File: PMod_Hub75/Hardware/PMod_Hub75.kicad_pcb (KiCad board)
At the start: 2 copper layers, 45 x 40 mm, 16 parts, among them IC1 SN74LVC8T245DWR, IC2 SN74LVC8T245DWR, J1 Conn_02x06_Counter_Clockwise, J2 Conn_02x06_Counter_Clockwise, J3 Conn_02x08_Counter_Clockwise

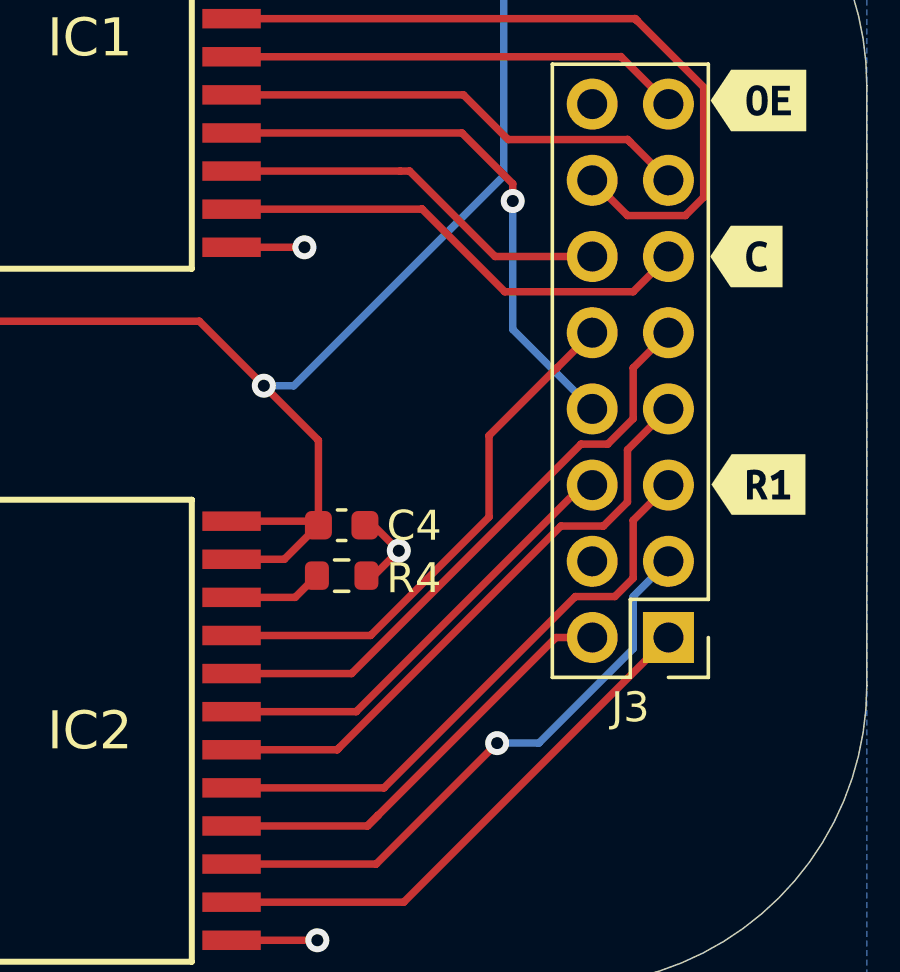
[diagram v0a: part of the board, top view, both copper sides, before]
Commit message: Fix design rules issues in pcb
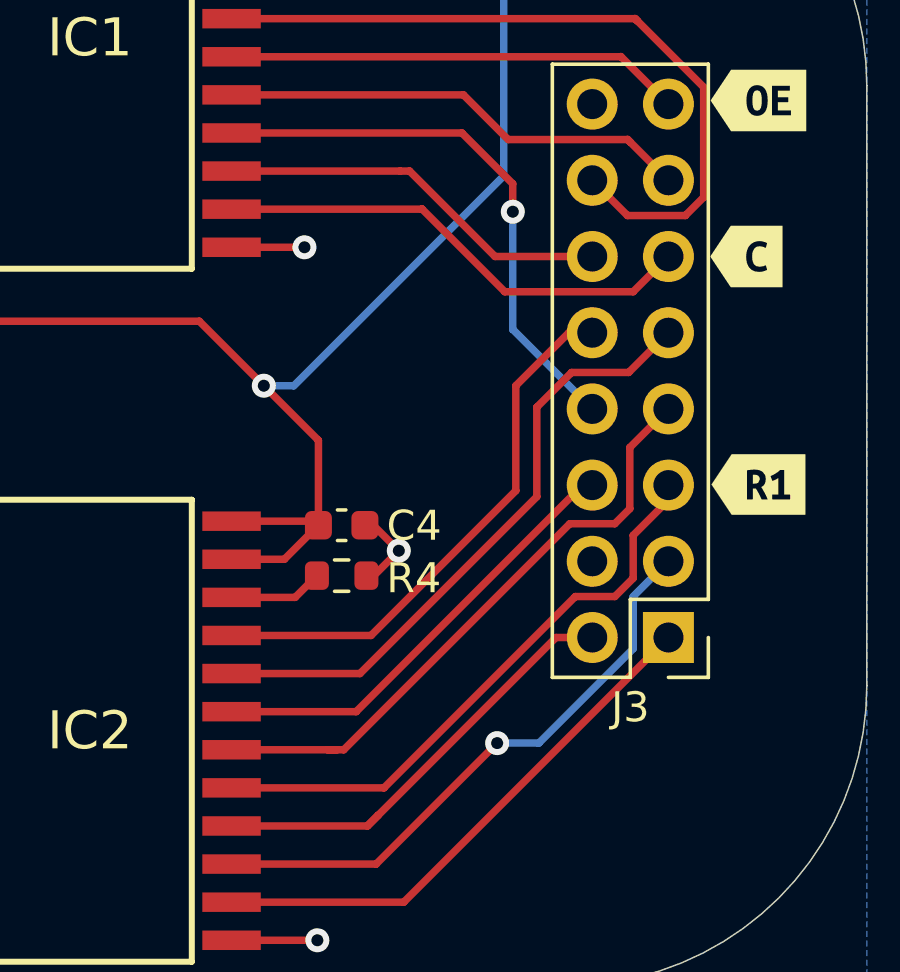
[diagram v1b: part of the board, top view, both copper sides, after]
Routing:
- net Out_A: track 20.3 -> 21.0 mm
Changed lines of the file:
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@@
   (segment (start 146.505 96.575) (end 148.1975 98.2675) (width 0.25) (layer "F.Cu") (net 9))
   (segment (start 138.825 96.575) (end 146.505 96.575) (width 0.25) (layer "F.Cu") (net 9))
-  (segment (start 148.1975 98.2675) (end 148.1975 98.842499) (width 0.25) (layer "F.Cu") (net 9))
-  (via (at 148.1975 98.842499) (size 0.8) (drill 0.4) (layers "F.Cu" "B.Cu") (net 9))
-  (segment (start 148.1975 103.122499) (end 148.1975 98.842499) (width 0.25) (layer "B.Cu") (net 9))
+  (segment (start 148.1975 98.2675) (end 148.1975 99.1975) (width 0.25) (layer "F.Cu") (net 9))
+  (segment (start 148.1975 99.1975) (end 148.2 99.2) (width 0.25) (layer "F.Cu") (net 9))
+  (via (at 148.2 99.2) (size 0.8) (drill 0.4) (layers "F.Cu" "B.Cu") (net 9))
+  (segment (start 148.2 99.2) (end 148.2 103.119999) (width 0.25) (layer "B.Cu") (net 9))
   (segment (start 150.8475 105.772499) (end 148.1975 103.122499) (width 0.25) (layer "B.Cu") (net 9))
+  (segment (start 148.2 103.119999) (end 148.1975 103.122499) (width 0.25) (layer "B.Cu") (net 9))
   (segment (start 147.6075 100.692499) (end 144.760001 97.845) (width 0.25) (layer "F.Cu") (net 10))
   (segment (start 144.760001 97.845) (end 144.445 97.845) (width 0.25) (layer "F.Cu") (net 10))
@@
   (segment (start 138.825 112.055) (end 140.945 112.055) (width 0.25) (layer "F.Cu") (net 19))
   (segment (start 140.945 112.055) (end 141.67 111.33) (width 0.25) (layer "F.Cu") (net 19))
-  (segment (start 143.460279 113.325) (end 147.4075 109.377779) (width 0.25) (layer "F.Cu") (net 20))
-  (segment (start 149.662499 104.4075) (end 149.672499 104.4075) (width 0.25) (layer "F.Cu") (net 20))
-  (segment (start 147.4075 109.377779) (end 147.4075 106.662499) (width 0.25) (layer "F.Cu") (net 20))
-  (segment (start 149.672499 104.4075) (end 150.8475 103.232499) (width 0.25) (layer "F.Cu") (net 20))
-  (segment (start 147.4075 106.662499) (end 149.662499 104.4075) (width 0.25) (layer "F.Cu") (net 20))
-  (segment (start 138.825 113.325) (end 143.460279 113.325) (width 0.25) (layer "F.Cu") (net 20))
-  (segment (start 142.825997 114.595) (end 138.825 114.595) (width 0.25) (layer "F.Cu") (net 21))
-  (segment (start 151.362989 106.94701) (end 150.473987 106.94701) (width 0.25) (layer "F.Cu") (net 21))
-  (segment (start 153.3875 103.232499) (end 152.212499 104.4075) (width 0.25) (layer "F.Cu") (net 21))
-  (segment (start 152.212499 106.0975) (end 151.362989 106.94701) (width 0.25) (layer "F.Cu") (net 21))
-  (segment (start 152.212499 104.4075) (end 152.212499 106.0975) (width 0.25) (layer "F.Cu") (net 21))
-  (segment (start 150.473987 106.94701) (end 142.825997 114.595) (width 0.25) (layer "F.Cu") (net 21))
+  (segment (start 143.475 113.325) (end 148.3 108.5) (width 0.25) (layer "F.Cu") (net 20))
+  (segment (start 148.3 108.5) (end 148.3 105) (width 0.25) (layer "F.Cu") (net 20))
+  (segment (start 148.3 105) (end 150.067501 103.232499) (width 0.25) (layer "F.Cu") (net 20))
+  (segment (start 138.825 113.325) (end 143.475 113.325) (width 0.25) (layer "F.Cu") (net 20))
+  (segment (start 150.067501 103.232499) (end 150.8475 103.232499) (width 0.25) (layer "F.Cu") (net 20))
+  (segment (start 149 108.7) (end 149 105.715716) (width 0.25) (layer "F.Cu") (net 21))
+  (segment (start 138.825 114.595) (end 143.105 114.595) (width 0.25) (layer "F.Cu") (net 21))
+  (segment (start 143.105 114.595) (end 149 108.7) (width 0.25) (layer "F.Cu") (net 21))
+  (segment (start 150.157858 104.557858) (end 152.062141 104.557858) (width 0.25) (layer "F.Cu") (net 21))
+  (segment (start 152.062141 104.557858) (end 153.3875 103.232499) (width 0.25) (layer "F.Cu") (net 21))
+  (segment (start 149 105.715716) (end 150.157858 104.557858) (width 0.25) (layer "F.Cu") (net 21))
   (segment (start 150.53109 108.312499) (end 142.978589 115.865) (width 0.25) (layer "F.Cu") (net 22))
   (segment (start 150.8475 108.312499) (end 150.53109 108.312499) (width 0.25) (layer "F.Cu") (net 22))
   (segment (start 142.978589 115.865) (end 138.825 115.865) (width 0.25) (layer "F.Cu") (net 22))
-  (segment (start 142.345 117.135) (end 138.825 117.135) (width 0.25) (layer "F.Cu") (net 23))
-  (segment (start 142.39 117.09) (end 142.345 117.135) (width 0.25) (layer "F.Cu") (net 23))
-  (segment (start 152.022501 107.137498) (end 152.022501 108.8765) (width 0.25) (layer "F.Cu") (net 23))
-  (segment (start 149.802501 109.677498) (end 142.39 117.09) (width 0.25) (layer "F.Cu") (net 23))
-  (segment (start 142.39 117.09) (end 142.3525 117.127499) (width 0.25) (layer "F.Cu") (net 23))
-  (segment (start 152.022501 108.8765) (end 151.221503 109.677498) (width 0.25) (layer "F.Cu") (net 23))
-  (segment (start 153.3875 105.772499) (end 152.022501 107.137498) (width 0.25) (layer "F.Cu") (net 23))
-  (segment (start 151.221503 109.677498) (end 149.802501 109.677498) (width 0.25) (layer "F.Cu") (net 23))
-  (segment (start 150.283499 112.0275) (end 143.905999 118.405) (width 0.25) (layer "F.Cu") (net 24))
-  (segment (start 152.212499 109.4875) (end 152.212499 111.4165) (width 0.25) (layer "F.Cu") (net 24))
-  (segment (start 151.601499 112.0275) (end 150.283499 112.0275) (width 0.25) (layer "F.Cu") (net 24))
-  (segment (start 143.905999 118.405) (end 138.825 118.405) (width 0.25) (layer "F.Cu") (net 24))
-  (segment (start 152.212499 111.4165) (end 151.601499 112.0275) (width 0.25) (layer "F.Cu") (net 24))
-  (segment (start 153.3875 108.312499) (end 152.212499 109.4875) (width 0.25) (layer "F.Cu") (net 24))
+  (segment (start 142.565 117.135) (end 142.035 117.135) (width 0.25) (layer "F.Cu") (net 23))
+  (segment (start 152.1 109.1) (end 152.1 107.06) (width 0.25) (layer "F.Cu") (net 23))
+  (segment (start 152.1 107.06) (end 153.3875 105.772499) (width 0.25) (layer "F.Cu") (net 23))
+  (segment (start 142.345 117.135) (end 142.035 117.135) (width 0.25) (layer "F.Cu") (net 23))
+  (segment (start 151.6 109.6) (end 152.1 109.1) (width 0.25) (layer "F.Cu") (net 23))
+  (segment (start 150.1 109.6) (end 142.565 117.135) (width 0.25) (layer "F.Cu") (net 23))
+  (segment (start 150.1 109.6) (end 151.6 109.6) (width 0.25) (layer "F.Cu") (net 23))
+  (segment (start 142.035 117.135) (end 138.825 117.135) (width 0.25) (layer "F.Cu") (net 23))
+  (segment (start 151.601499 112.0275) (end 152.212499 111.4165) (width 0.25) (layer "F.Cu") (net 24))
+  (segment (start 153.3875 108.8125) (end 153.3875 108.312499) (width 0.25) (layer "F.Cu") (net 24))
+  (segment (start 150.283499 112.0275) (end 151.601499 112.0275) (width 0.25) (layer "F.Cu") (net 24))
+  (segment (start 152.212499 109.987501) (end 153.3875 108.8125) (width 0.25) (layer "F.Cu") (net 24))
+  (segment (start 138.825 118.405) (end 143.905999 118.405) (width 0.25) (layer "F.Cu") (net 24))
+  (segment (start 152.212499 111.4165) (end 152.212499 109.987501) (width 0.25) (layer "F.Cu") (net 24))
+  (segment (start 143.905999 118.405) (end 150.283499 112.0275) (width 0.25) (layer "F.Cu") (net 24))
   (segment (start 150.8475 113.392499) (end 149.6375 113.392499) (width 0.25) (layer "F.Cu") (net 25))
   (segment (start 138.825 119.675) (end 143.355 119.675) (width 0.25) (layer "F.Cu") (net 25))
